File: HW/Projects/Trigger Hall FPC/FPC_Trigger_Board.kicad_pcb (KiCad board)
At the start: 2 copper layers, 20.3 x 17.9 mm, 8 parts, among them U1 HAL4395, U2 HAL4395

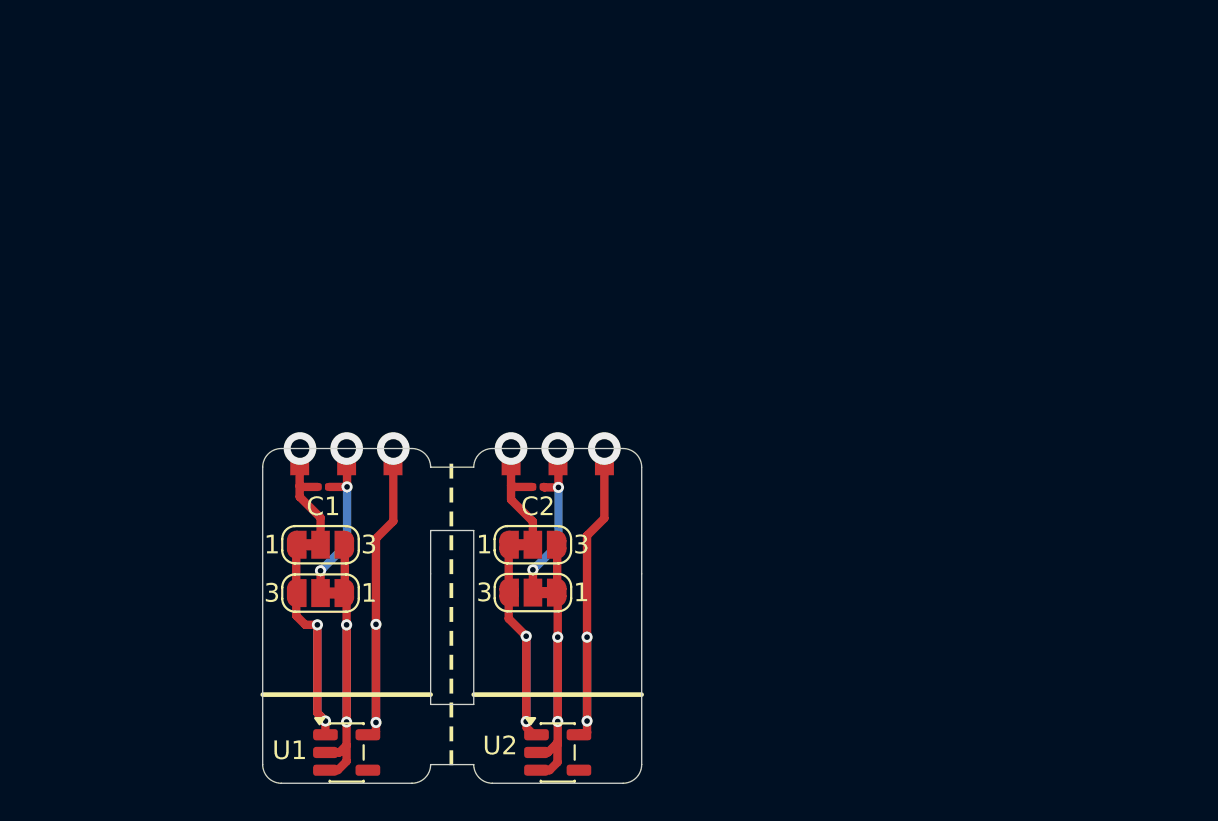
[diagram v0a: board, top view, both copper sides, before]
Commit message: R5/S1 Updates
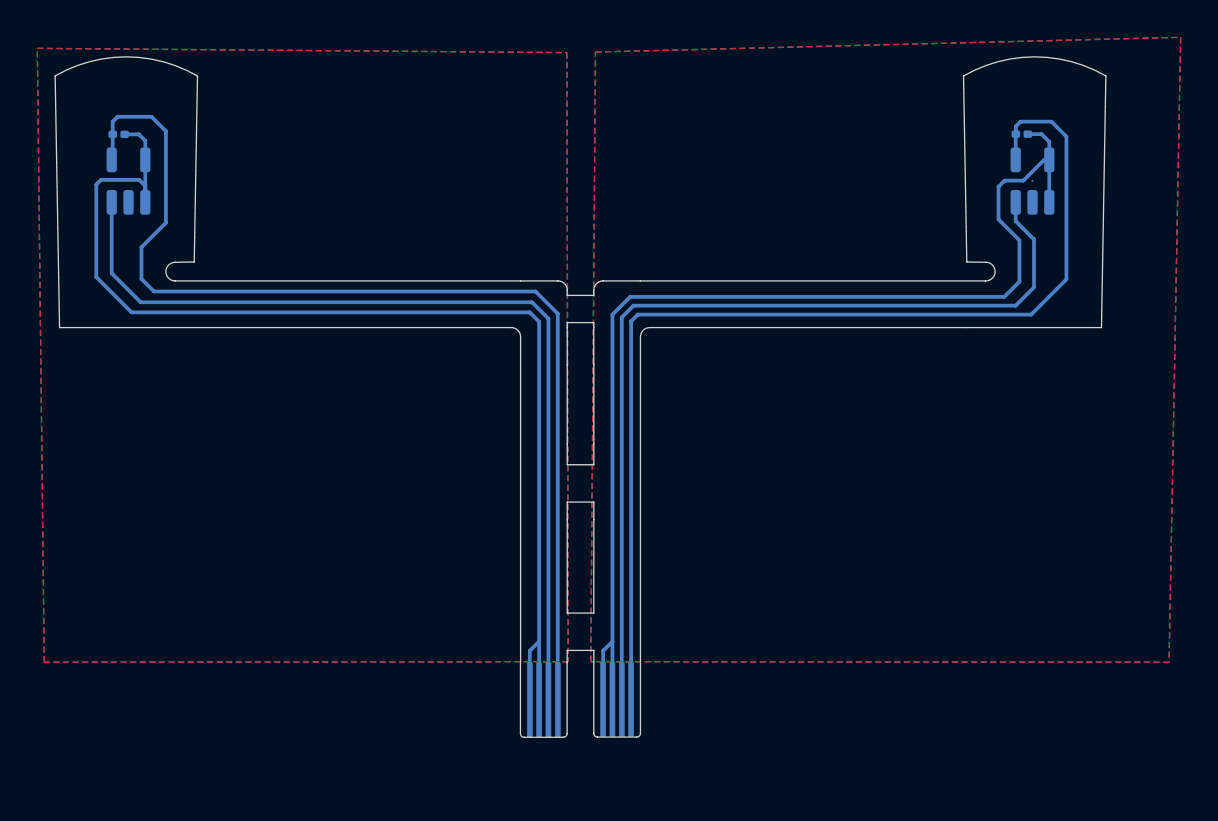
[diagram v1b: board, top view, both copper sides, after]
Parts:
- removed JP1, JP2, JP3, JP4: SolderJumper_3_Bridged12, Jumper:SolderJumper-3_P1.3mm_Bridged12_RoundedPad1.0x1.5mm_NumberLabels
- added J1: Conn_01x04_Pin, hhl:505110-0492 Ribbon, F.Cu at (226.6, 160.2)
- added J2: Conn_01x04_Pin, hhl:505110-0492 Ribbon, F.Cu at (230.6, 160.2)
- C1, C2: moved to B.Cu
- U1, U2: footprint Package_TO_SOT_SMD:SOT-23-5 -> hhl:SOT-23-5L; moved to B.Cu
- moved U2 39.8 mm to (252.8, 132.4), turned to 90 degrees
- moved U1 32.8 mm to (204.4, 132.4), turned to 90 degrees
- moved C2 32.1 mm to (252.2, 129.9)
- moved C1 21.8 mm to (203.8, 129.9)
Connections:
- C1 pad 1: PAD_2L -> GNDL
- C1 pad 2: PAD_1L -> +3V3L
- C2 pad 1: PAD_2R -> GND
- C2 pad 2: PAD_1R -> +3V3
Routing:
- net GNDL: track 19.5 -> 61.6 mm, vias 2 -> 0
- net +3V3: track 15.2 -> 57.1 mm, vias 2 -> 0
- net GND: track 18.8 -> 59.9 mm, vias 2 -> 0
- net +3V3L: track 16.5 -> 57.6 mm, vias 2 -> 0
- net ADC_1: track 20.3 -> 48.2 mm, vias 3 -> 0
- net ADC_0: track 20.8 -> 48.6 mm, vias 3 -> 0
- net PAD_2L: track 8.65 -> 0.00 mm, vias 3 -> 0
- net PAD_2R: track 8.44 -> 0.00 mm, vias 3 -> 0
- net PAD_1R: track 6.14 -> 0.00 mm, vias 1 -> 0
- net PAD_1L: track 5.94 -> 0.00 mm, vias 1 -> 0
- added copper zone on B.Cu, net GND
- added copper zone on F.Cu, net GND
- added copper zone on B.Cu, net GNDL
- added copper zone on F.Cu, net GNDL
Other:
- board size 20.3 x 17.9 mm -> 56.3 x 32.5 mm
